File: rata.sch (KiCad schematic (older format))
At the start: 2 parts

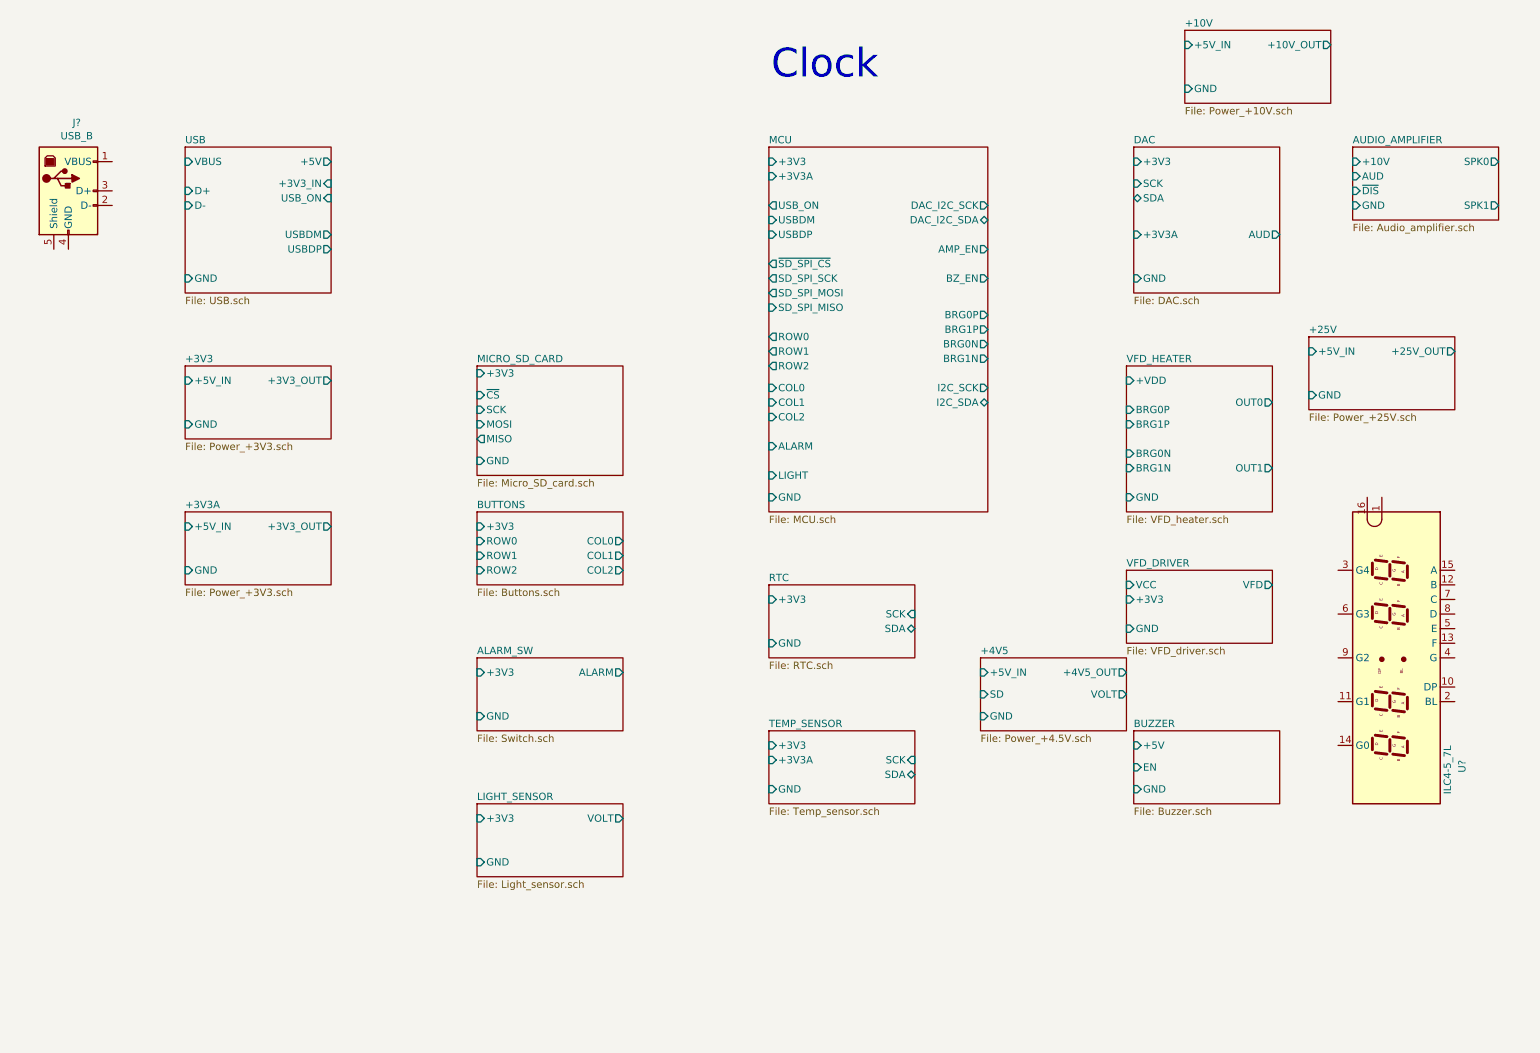
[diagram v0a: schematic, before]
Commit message: Add files via upload
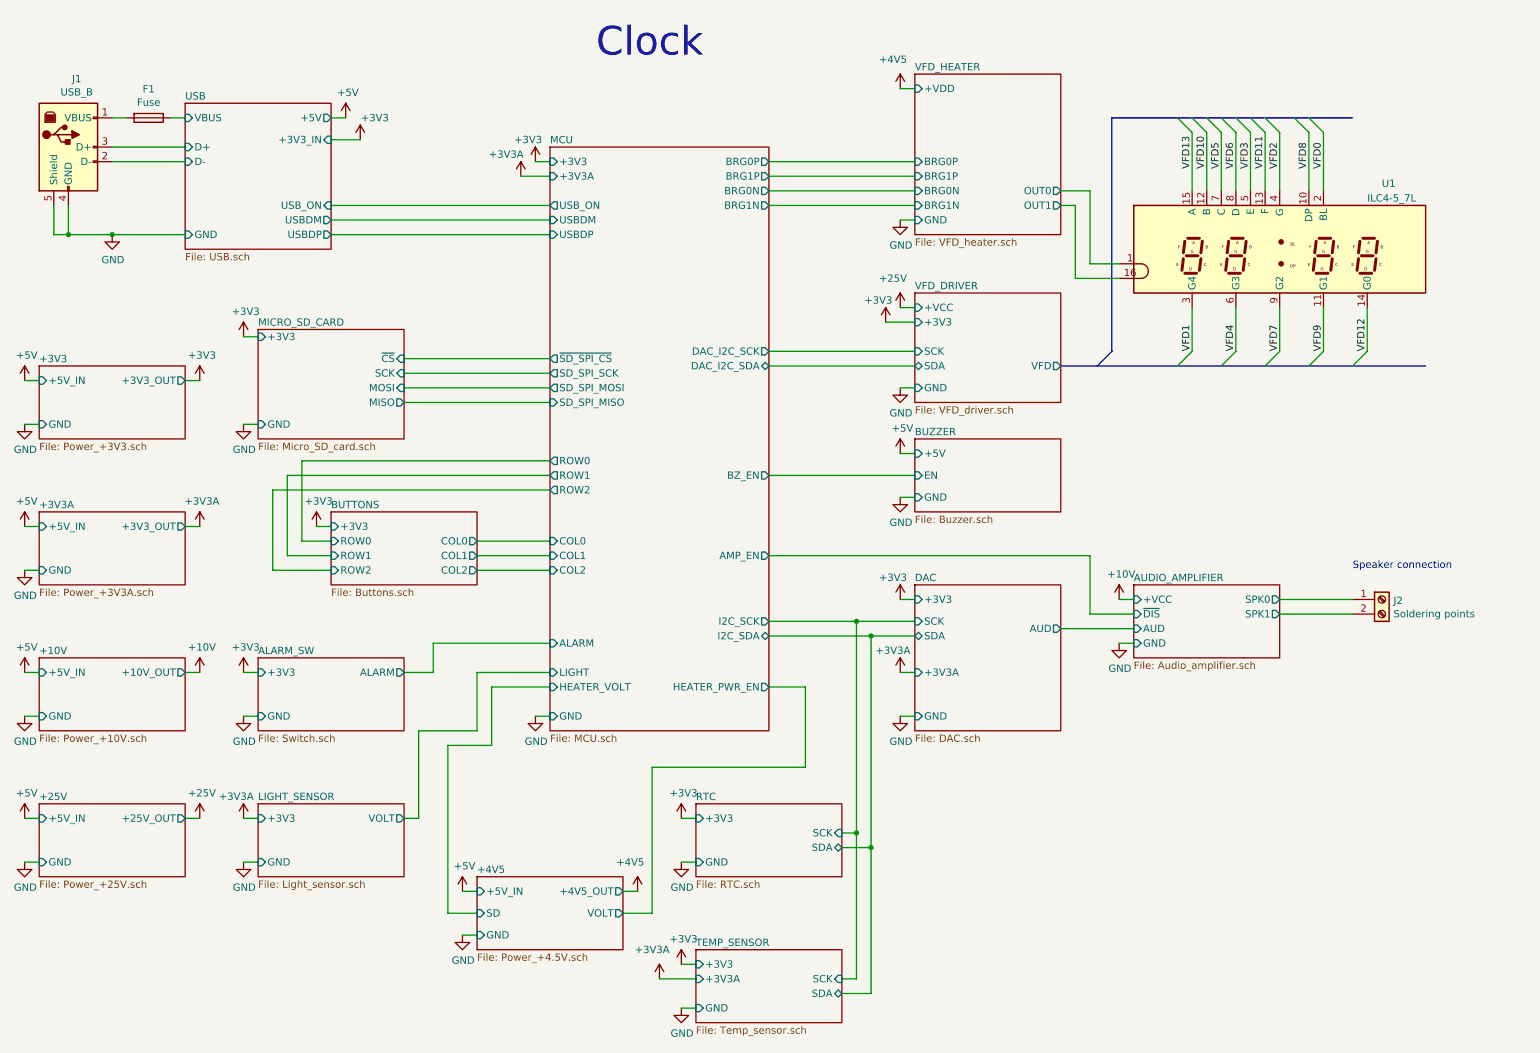
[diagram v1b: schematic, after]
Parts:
- added F1: Fuse, symbol Device:Fuse
- added J2: Soldering points, symbol Connector:Screw_Terminal_01x02
- gave numbers to parts that had none: 2
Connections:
- net AUDIO_AMPLIFIER/SPK0: now also J2.1 (Pin_1)
- net AUDIO_AMPLIFIER/SPK1: now also J2.2 (Pin_2)
- net USB/D+: now also J1.3 (D+)
- net USB/D-: now also J1.2 (D-)
- net USB/VBUS: now also F1.1
- net VFD_HEATER/OUT0: now also U1.1
- net VFD_HEATER/OUT1: now also U1.16
- net VFD8: now reaches U1.10 (DP)
- net VFD9: now reaches U1.11 (G1)
- net VFD10: now reaches U1.12 (B)
- net VFD11: now reaches U1.13 (F)
- net VFD12: now reaches U1.14 (G0)
- net VFD13: now reaches U1.15 (A)
- net VFD0: now reaches U1.2 (BL)
- net VFD1: now reaches U1.3 (G4)
- net VFD2: now reaches U1.4 (G)
- net VFD3: now reaches U1.5 (E)
- net VFD4: now reaches U1.6 (G3)
- net VFD5: now reaches U1.7 (C)
- net VFD6: now reaches U1.8 (D)
- net VFD7: now reaches U1.9 (G2)
- net at J1.1 (VBUS): now also F1.2
- net GND: now reaches J1.4 (GND)
- net GND: now also J1.5 (Shield)
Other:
- note added: "Speaker connection"
- moved on the sheet: J1, U1
